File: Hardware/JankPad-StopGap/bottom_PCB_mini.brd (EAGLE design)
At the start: 110.5 x 67.5 mm, 19 parts, among them X1 STEREOJACK

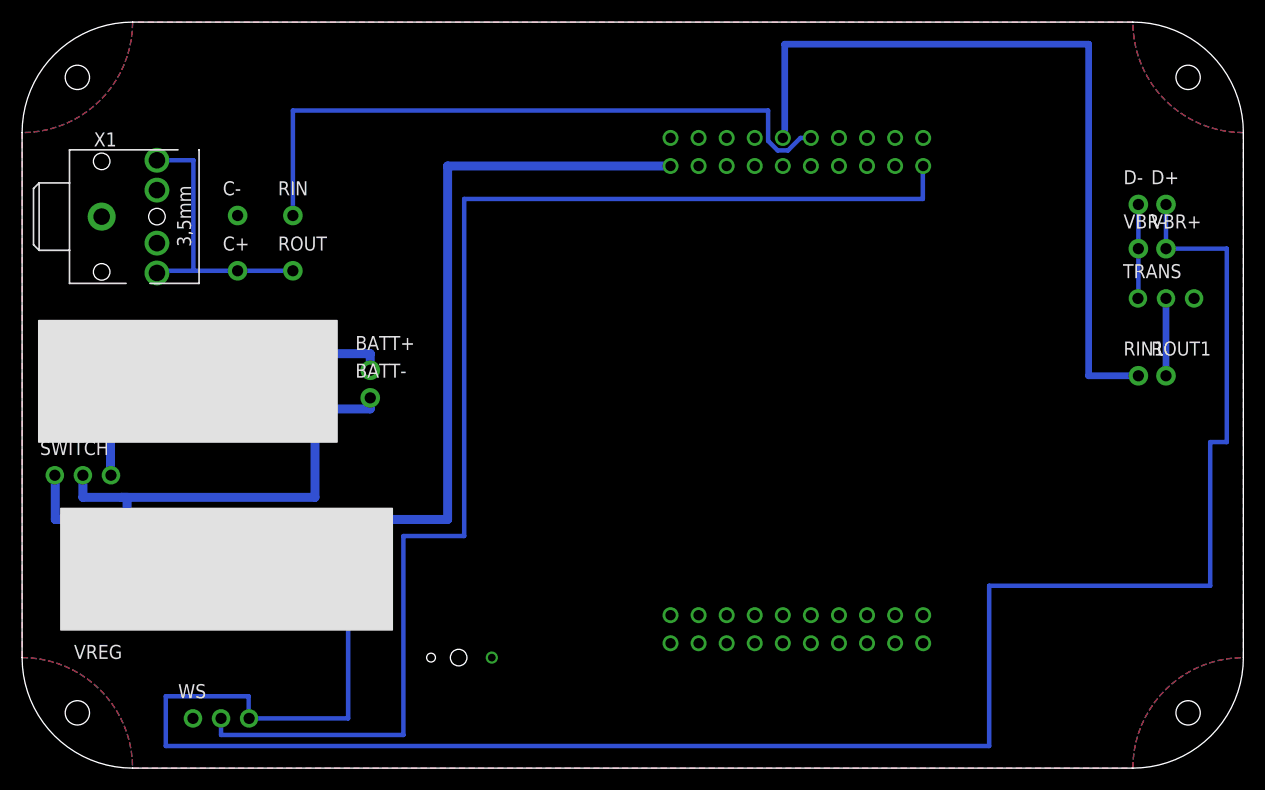
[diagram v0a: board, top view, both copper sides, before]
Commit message: bugs everywhere
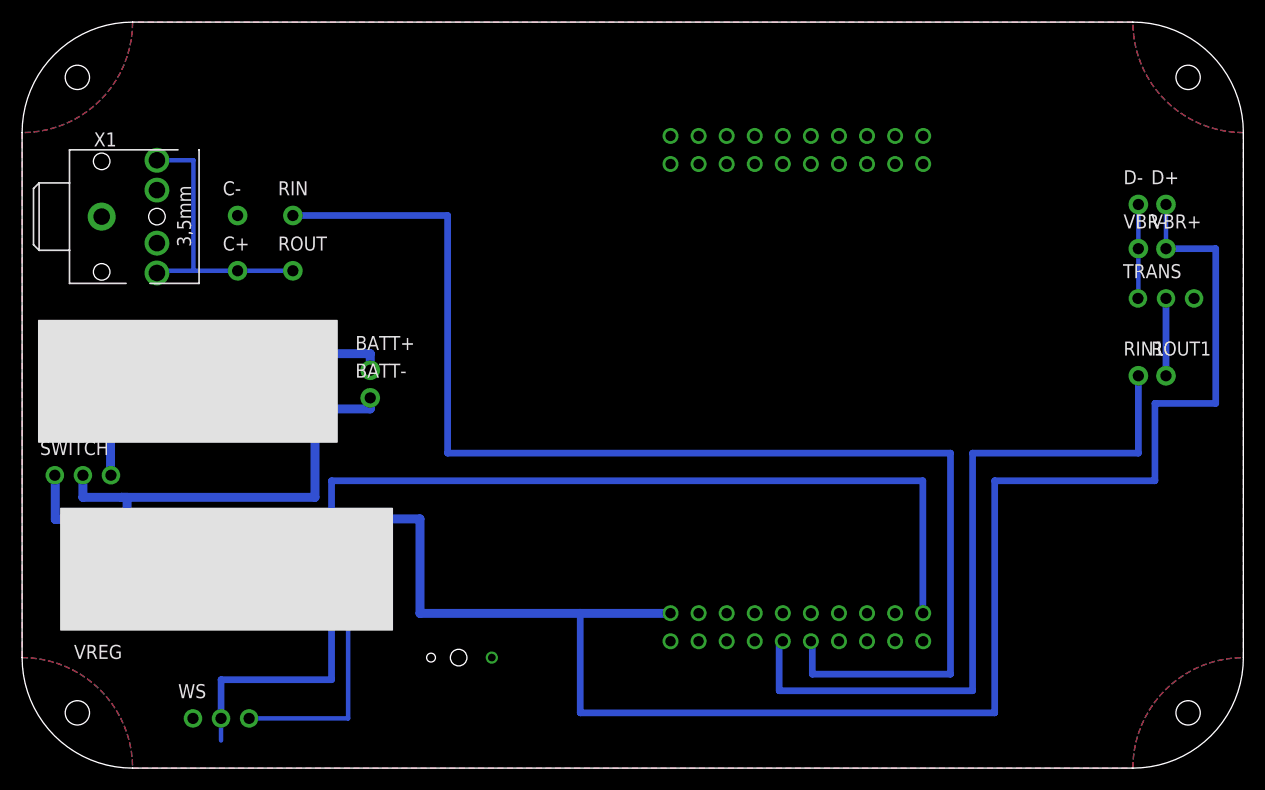
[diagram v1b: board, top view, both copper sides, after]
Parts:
- moved LAUNCHPAD 60.8 mm to (67.6, 3.86), flipped to the bottom, turned to 270 degrees
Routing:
- net N$8: track 252.8 -> 181.8 mm
- net N$10: track 59.9 -> 116.6 mm
- net N$9: track 116.5 -> 99.0 mm
- net N$11: track 70.7 -> 65.8 mm
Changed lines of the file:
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@@
 </autorouter>
 <elements>
-<element name="LAUNCHPAD" library="TM4C" package="1_05X2MM" value="TM4CTM4C" x="67.56" y="64.64" rot="R90"/>
+<element name="LAUNCHPAD" library="TM4C" package="1_05X2MM" value="TM4CTM4C" x="67.56" y="3.86" rot="MR270"/>
 <element name="X1" library="adafruit" package="STX3100" value="STEREOJACK" x="4.5" y="50"/>
 <element name="WS" library="adafruit" package="1X03-CLEANBIG" value="" x="18" y="4.5"/>
@@
 <wire x1="29.5" y1="22.5" x2="32" y2="22.5" width="0.4064" layer="16"/>
 <wire x1="32" y1="22.55" x2="32" y2="22.5" width="0.4064" layer="16"/>
-<wire x1="58.67" y1="54.48" x2="38.5" y2="54.48" width="0.8128" layer="16"/>
-<wire x1="38.5" y1="54.48" x2="38.5" y2="22.5" width="0.8128" layer="16"/>
-<wire x1="38.5" y1="22.5" x2="32" y2="22.5" width="0.8128" layer="16"/>
-<wire x1="32" y1="22.5" x2="32" y2="22.55" width="0.8128" layer="16"/>
-<wire x1="20.54" y1="4.5" x2="20.5" y2="4.5" width="0.4064" layer="16"/>
-<wire x1="20.5" y1="4.5" x2="20.5" y2="6.5" width="0.4064" layer="16"/>
-<wire x1="20.5" y1="6.5" x2="13" y2="6.5" width="0.4064" layer="16"/>
-<wire x1="13" y1="6.5" x2="13" y2="2" width="0.4064" layer="16"/>
-<wire x1="13" y1="2" x2="87.5" y2="2" width="0.4064" layer="16"/>
-<wire x1="87.5" y1="2" x2="87.5" y2="16.5" width="0.4064" layer="16"/>
-<wire x1="87.5" y1="16.5" x2="107.5" y2="16.5" width="0.4064" layer="16"/>
-<wire x1="107.5" y1="29.5" x2="109" y2="29.5" width="0.4064" layer="16"/>
-<wire x1="109" y1="29.5" x2="109" y2="47" width="0.4064" layer="16"/>
-<wire x1="109" y1="47" x2="103.5" y2="47" width="0.4064" layer="16"/>
-<wire x1="107.5" y1="16.5" x2="107.5" y2="29.5" width="0.4064" layer="16"/>
+<wire x1="32" y1="22.55" x2="36" y2="22.55" width="0.8128" layer="16"/>
+<wire x1="50.5" y1="14" x2="36" y2="14" width="0.8128" layer="16"/>
+<wire x1="50.5" y1="14" x2="58.67" y2="14" width="0.8128" layer="16"/>
+<wire x1="58.67" y1="14" x2="58.67" y2="14.02" width="0.8128" layer="16"/>
+<wire x1="36" y1="22.55" x2="36" y2="14" width="0.8128" layer="16"/>
+<wire x1="103.5" y1="47" x2="108" y2="47" width="0.6096" layer="16"/>
+<wire x1="108" y1="47" x2="108" y2="33" width="0.6096" layer="16"/>
+<wire x1="108" y1="33" x2="102.5" y2="33" width="0.6096" layer="16"/>
+<wire x1="102.5" y1="33" x2="102.5" y2="26" width="0.6096" layer="16"/>
+<wire x1="102.5" y1="26" x2="88" y2="26" width="0.6096" layer="16"/>
+<wire x1="88" y1="26" x2="88" y2="5" width="0.6096" layer="16"/>
+<wire x1="88" y1="5" x2="50.5" y2="5" width="0.6096" layer="16"/>
+<wire x1="50.5" y1="5" x2="50.5" y2="14" width="0.6096" layer="16"/>
 </signal>
 <signal name="N$9">
 <contactref element="WS" pad="2"/>
 <contactref element="LAUNCHPAD" pad="PF1"/>
-<wire x1="81.53" y1="54.48" x2="81.5" y2="54.48" width="0.4064" layer="16"/>
-<wire x1="81.5" y1="54.48" x2="81.5" y2="51.5" width="0.4064" layer="16"/>
-<wire x1="81.5" y1="51.5" x2="40" y2="51.5" width="0.4064" layer="16"/>
-<wire x1="40" y1="21" x2="34.5" y2="21" width="0.4064" layer="16"/>
-<wire x1="34.5" y1="21" x2="34.5" y2="3" width="0.4064" layer="16"/>
-<wire x1="34.5" y1="3" x2="18" y2="3" width="0.4064" layer="16"/>
-<wire x1="18" y1="3" x2="18" y2="4.5" width="0.4064" layer="16"/>
-<wire x1="40" y1="51.5" x2="40" y2="21" width="0.4064" layer="16"/>
+<wire x1="18" y1="4.5" x2="18" y2="2.5" width="0.4064" layer="16"/>
+<wire x1="81.53" y1="14" x2="81.53" y2="14.02" width="0.4064" layer="16"/>
+<wire x1="81.53" y1="14.02" x2="81.5" y2="14.02" width="0.6096" layer="16"/>
+<wire x1="81.5" y1="14.02" x2="81.5" y2="26" width="0.6096" layer="16"/>
+<wire x1="81.5" y1="26" x2="28" y2="26" width="0.6096" layer="16"/>
+<wire x1="28" y1="26" x2="28" y2="8" width="0.6096" layer="16"/>
+<wire x1="28" y1="8" x2="18" y2="8" width="0.6096" layer="16"/>
+<wire x1="18" y1="8" x2="18" y2="4.5" width="0.6096" layer="16"/>
 </signal>
 <signal name="N$10">
 <contactref element="LAUNCHPAD" pad="PE5"/>
 <contactref element="RIN" pad="1"/>
-<wire x1="69.2981875" y1="55.8897" x2="68.3618125" y2="55.8897" width="0.4064" layer="16"/>
-<wire x1="71.37" y1="57.02" x2="70.4284875" y2="57.02" width="0.4064" layer="16"/>
-<wire x1="70.4284875" y1="57.02" x2="69.2981875" y2="55.8897" width="0.4064" layer="16"/>
-<wire x1="68.3618125" y1="55.8897" x2="67.5" y2="56.7515125" width="0.4064" layer="16"/>
-<wire x1="67.5" y1="56.7515125" x2="67.5" y2="59.5" width="0.4064" layer="16"/>
-<wire x1="67.5" y1="59.5" x2="24.5" y2="59.5" width="0.4064" layer="16"/>
-<wire x1="24.5" y1="59.5" x2="24.5" y2="50" width="0.4064" layer="16"/>
+<wire x1="71.37" y1="11.48" x2="71.5" y2="11.48" width="0.6096" layer="16"/>
+<wire x1="71.5" y1="11.48" x2="71.5" y2="8.5" width="0.6096" layer="16"/>
+<wire x1="71.5" y1="8.5" x2="84" y2="8.5" width="0.6096" layer="16"/>
+<wire x1="84" y1="8.5" x2="84" y2="28.5" width="0.6096" layer="16"/>
+<wire x1="84" y1="28.5" x2="38.5" y2="28.5" width="0.6096" layer="16"/>
+<wire x1="38.5" y1="28.5" x2="38.5" y2="50" width="0.6096" layer="16"/>
+<wire x1="38.5" y1="50" x2="24.5" y2="50" width="0.6096" layer="16"/>
 </signal>
 <signal name="N$7">
@@
 <contactref element="RIN1" pad="1"/>
 <contactref element="LAUNCHPAD" pad="PE4"/>
-<wire x1="68.83" y1="57.02" x2="69" y2="57.02" width="0.6096" layer="16"/>
-<wire x1="69" y1="57.02" x2="69" y2="65.5" width="0.6096" layer="16"/>
-<wire x1="69" y1="65.5" x2="96.5" y2="65.5" width="0.6096" layer="16"/>
-<wire x1="96.5" y1="65.5" x2="96.5" y2="35.5" width="0.6096" layer="16"/>
-<wire x1="96.5" y1="35.5" x2="101" y2="35.5" width="0.6096" layer="16"/>
+<wire x1="68.83" y1="11.48" x2="68.5" y2="11.48" width="0.6096" layer="16"/>
+<wire x1="68.5" y1="11.48" x2="68.5" y2="7" width="0.6096" layer="16"/>
+<wire x1="68.5" y1="7" x2="86" y2="7" width="0.6096" layer="16"/>
+<wire x1="86" y1="7" x2="86" y2="28.5" width="0.6096" layer="16"/>
+<wire x1="86" y1="28.5" x2="101" y2="28.5" width="0.6096" layer="16"/>
+<wire x1="101" y1="28.5" x2="101" y2="35.5" width="0.6096" layer="16"/>
 </signal>
 <signal name="N$13">
